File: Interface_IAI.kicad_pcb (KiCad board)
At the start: 2 copper layers, 98.8 x 120 mm, 42 parts, among them J1 +24V, J2 ADWIN_DIO32, J3 SCON_FEEDBACK, J4 SCON_PULSE, J5 SCON_PIO, J6 ADWin CO4-T, U1 AM26LS31, U2 AM26LS32, U3 TBD62783APG, U4 TSR1-2450E

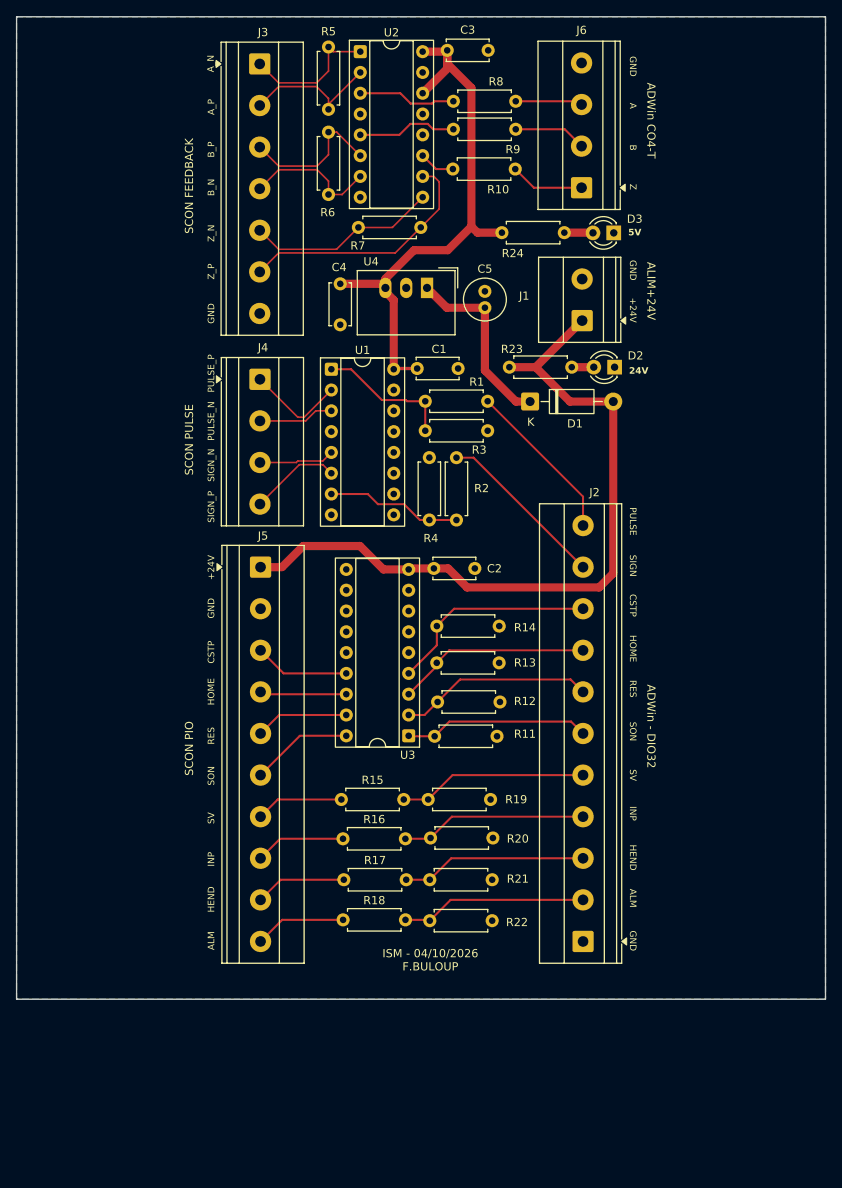
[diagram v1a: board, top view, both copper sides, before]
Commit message: Update gerber files
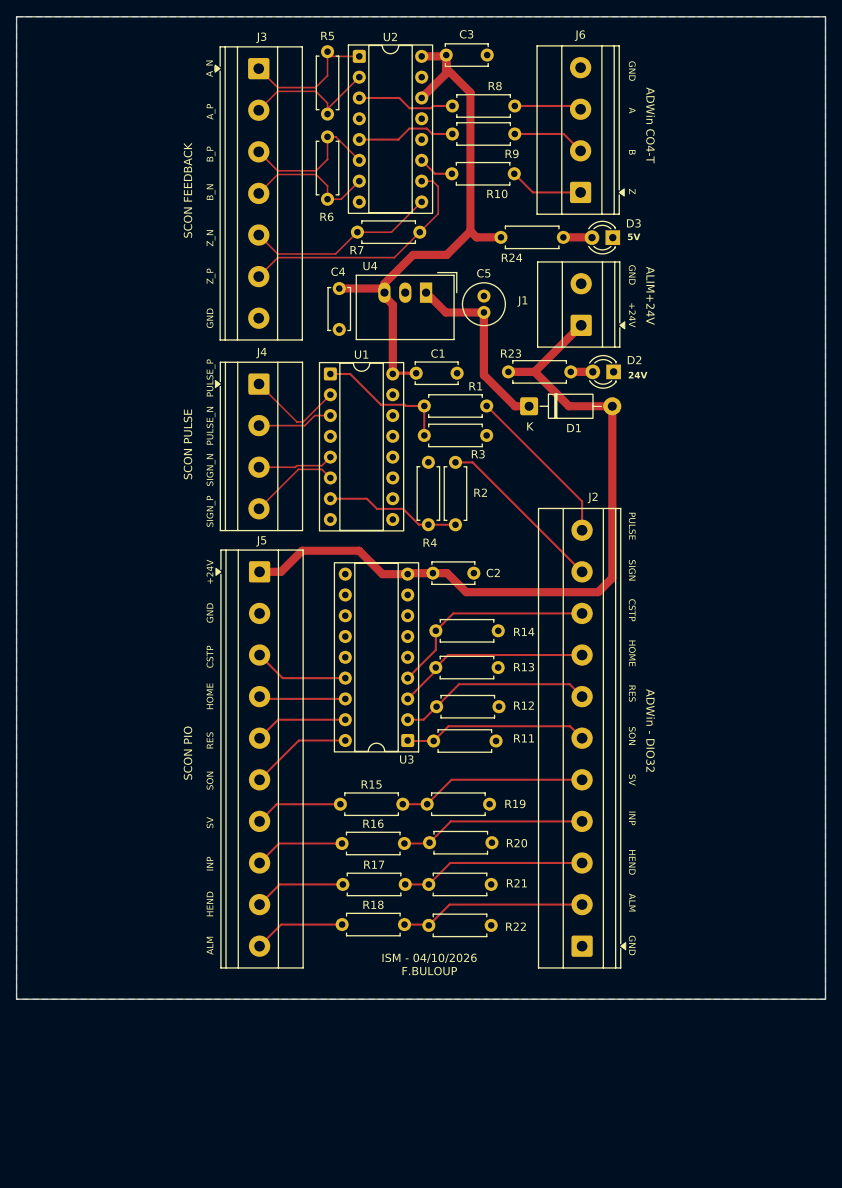
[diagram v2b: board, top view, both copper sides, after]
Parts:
- moved C4 0.59 mm to (89.4, 83.2)
- moved C5 0.59 mm to (107.1, 86.1)
- moved J6 0.59 mm to (118.9, 71.5)
- moved R24 0.59 mm to (109.2, 77.0)
- moved R4 0.59 mm to (100.3, 112.1)
- moved U1 0.59 mm to (88.3, 93.7)
- moved C1 0.59 mm to (98.8, 93.6)
- moved C2 0.59 mm to (100.9, 118.0)
- moved C3 0.59 mm to (102.5, 54.7)
- moved D3 0.59 mm to (122.8, 77.0)
- moved R1 0.59 mm to (107.4, 97.6)
- moved R10 0.59 mm to (103.2, 69.2)
- moved R2 0.59 mm to (103.6, 104.5)
- moved R9 0.59 mm to (103.2, 64.3)
- moved U4 0.59 mm to (100.0, 83.7)
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
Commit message: Update Doc.
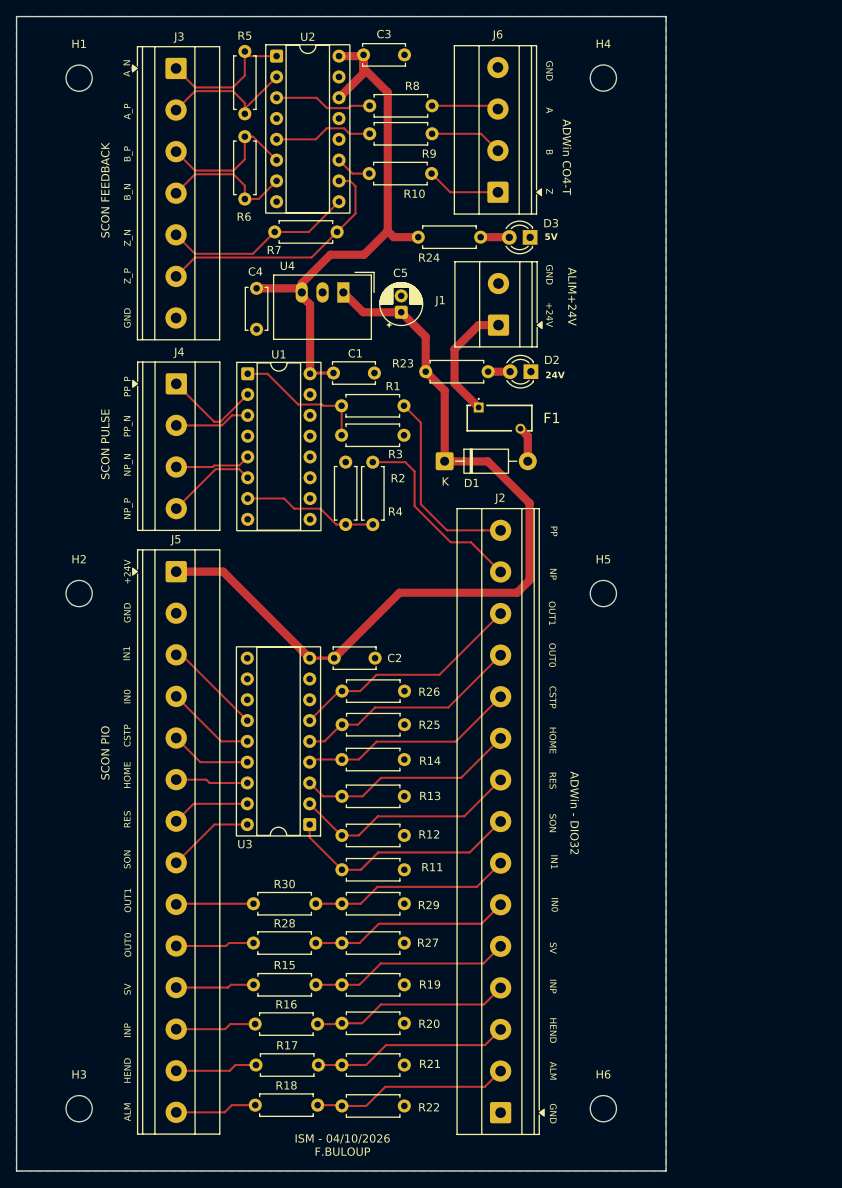
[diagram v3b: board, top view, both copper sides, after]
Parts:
- added F1: Polyfuse, MF-R050:MFR050, F.Cu at (106.4, 97.7)
- added H1: MountingHole, MountingHole:MountingHole_3.2mm_M3, F.Cu at (57.6, 57.5)
- added H2: MountingHole, MountingHole:MountingHole_3.2mm_M3, F.Cu at (57.6, 120.5)
- added H3: MountingHole, MountingHole:MountingHole_3.2mm_M3, F.Cu at (57.6, 183.4)
- added H4: MountingHole, MountingHole:MountingHole_3.2mm_M3, F.Cu at (121.7, 57.5)
- added H5: MountingHole, MountingHole:MountingHole_3.2mm_M3, F.Cu at (121.7, 120.5)
- added H6: MountingHole, MountingHole:MountingHole_3.2mm_M3, F.Cu at (121.7, 183.4)
- added R25: 10k, Resistor_THT:R_Axial_DIN0207_L6.3mm_D2.5mm_P7.62mm_Horizontal, F.Cu at (89.8, 136.5)
- added R26: 10k, Resistor_THT:R_Axial_DIN0207_L6.3mm_D2.5mm_P7.62mm_Horizontal, F.Cu at (89.8, 132.4)
- added R27: 2.2k, Resistor_THT:R_Axial_DIN0207_L6.3mm_D2.5mm_P7.62mm_Horizontal, F.Cu at (89.7, 163.2)
- added R28: 10k, Resistor_THT:R_Axial_DIN0207_L6.3mm_D2.5mm_P7.62mm_Horizontal, F.Cu at (78.9, 163.2)
- added R29: 2.2k, Resistor_THT:R_Axial_DIN0207_L6.3mm_D2.5mm_P7.62mm_Horizontal, F.Cu at (89.7, 158.4)
- added R30: 10k, Resistor_THT:R_Axial_DIN0207_L6.3mm_D2.5mm_P7.62mm_Horizontal, F.Cu at (78.9, 158.4)
- C5: footprint Capacitor_THT:C_Radial_D5.0mm_H11.0mm_P2.00mm -> Capacitor_THT:CP_Radial_D5.0mm_P2.00mm
- J2: value ADWIN_DIO32 -> Screw_Terminal_01x15; footprint TerminalBlock_Phoenix:TerminalBlock_Phoenix_MKDS-1,5-11-5.08_1x11_P5.08mm_Horizontal -> TerminalBlock_Phoenix:TerminalBlock_Phoenix_MKDS-1,5-15-5.08_1x15_P5.08mm_Horizontal
- J5: value SCON_PIO -> Screw_Terminal_01x14; footprint TerminalBlock_Phoenix:TerminalBlock_Phoenix_MKDS-1,5-10-5.08_1x10_P5.08mm_Horizontal -> TerminalBlock_Phoenix:TerminalBlock_Phoenix_MKDS-1,5-14-5.08_1x14_P5.08mm_Horizontal
- moved R20 24.5 mm to (89.7, 173.0)
- moved R17 24.5 mm to (79.2, 178.1)
- moved R21 24.5 mm to (89.7, 178.1)
- moved R22 24.5 mm to (89.7, 183.1)
- moved R15 24.5 mm to (78.9, 168.3)
- moved R16 24.5 mm to (79.1, 173.1)
- moved R18 24.5 mm to (79.2, 183.0)
- moved R19 24.4 mm to (89.7, 168.3)
- moved J2 22.6 mm to (109.1, 183.9)
- moved R12 19.5 mm to (89.7, 150.0)
- moved R14 19.5 mm to (89.7, 140.7)
- moved R13 19.5 mm to (89.7, 145.2)
- moved R11 19.3 mm to (89.7, 154.2)
- moved C2 15.9 mm to (88.8, 128.4)
- moved U3 15.8 mm to (85.8, 148.7)
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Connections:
- net /PULSE_N renamed /PP_N
- net /PULSE_P renamed /PP_P
- net /PULSE_TTL renamed /PP_TTL
- net /SIGN_N renamed /NP_N
- net /SIGN_P renamed /NP_P
- net /SIGN_TTL renamed /NP_TTL
- C5 pad 1: /VIN_REG -> +24V
- D1 pad 1: /VIN_REG -> +24V
- D1 pad 2: +24V -> Net-(D1-A)
- J1 pad 1: +24V -> Net-(J1-Pin_1)
- J2 pad 10: /DIO_SIGN -> /DIO_HOME
- J2 pad 11: /DIO_PULSE -> /DIO_CSTP
- J2 pad 6: /DIO_SON -> /DIO_IN0
- J2 pad 7: /DIO_RES -> /DIO_IN1
- J2 pad 8: /DIO_HOME -> /DIO_SON
- J2 pad 9: /DIO_CSTP -> /DIO_RES
- J5 pad 10: /SCON_ALM -> /SCON_OUT0
- J5 pad 3: /SCON_CSTP -> /SCON_IN1
- J5 pad 4: /SCON_HOME -> /SCON_IN0
- J5 pad 5: /SCON_RES -> /SCON_CSTP
- J5 pad 6: /SCON_SON -> /SCON_HOME
- J5 pad 7: /SCON_SV -> /SCON_RES
- J5 pad 8: /SCON_INP -> /SCON_SON
- J5 pad 9: /SCON_HEND -> /SCON_OUT1
- R1 pad 1: /DIO_PULSE -> /DIO_PP
- R2 pad 1: /DIO_SIGN -> /DIO_NP
- U3 pad 13: unconnected-(U3-O6-Pad13) -> /SCON_IN1
- U3 pad 14: unconnected-(U3-O5-Pad14) -> /SCON_IN0
- U3 pad 5: GND -> /DIO_OUT0
- U3 pad 6: GND -> /DIO_OUT1
- U4 pad 1: /VIN_REG -> +24V
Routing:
- net /DIO_OUT1: track 0.00 -> 28.4 mm
- net /DIO_OUT0: track 0.00 -> 27.6 mm
- net /DIO_IN1: track 0.00 -> 24.6 mm
- net /DIO_IN0: track 0.00 -> 24.5 mm
- net /DIO_PP: track 0.00 -> 23.9 mm
- net /DIO_NP: track 0.00 -> 23.7 mm
- net /VIN_REG: track 22.8 -> 0.00 mm
- net /DIO_SIGN: track 21.0 -> 0.00 mm
- net /DIO_PULSE: track 20.0 -> 0.00 mm
- net Net-(J1-Pin_1): track 0.00 -> 14.9 mm
- net +24V: track 90.5 -> 101.9 mm
- net /SCON_IN1: track 0.00 -> 11.4 mm
- net /SCON_IN0: track 0.00 -> 11.0 mm
- net /SCON_OUT0: track 0.00 -> 9.58 mm
- net /SCON_OUT1: track 0.00 -> 9.35 mm
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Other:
- board size 98.8 x 120 mm -> 79.3 x 141 mm
- board text added: "IN0"
- board text added: "IN1"
- board text added: "NP"
- board text added: "NP_N"
- board text added: "NP_P"
- board text added: "OUT0"
- board text added: "OUT1"
- board text added: "PP"
- board text added: "PP_N"
- board text added: "PP_P"
- board text removed: "PULSE"
- board text removed: "PULSE_N"
- board text removed: "PULSE_P"
- board text removed: "SIGN"
- board text removed: "SIGN_N"
- board text removed: "SIGN_P"
